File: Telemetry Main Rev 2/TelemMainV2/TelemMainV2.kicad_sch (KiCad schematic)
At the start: 19 parts, among them J1 8 pin ATM connector, J3 12 pin ATM connector, J4 SD to SPI (Molex nanofit), U3 NUCLEO-F446RE, U4 ISO1050DUB, U6 MCP6004

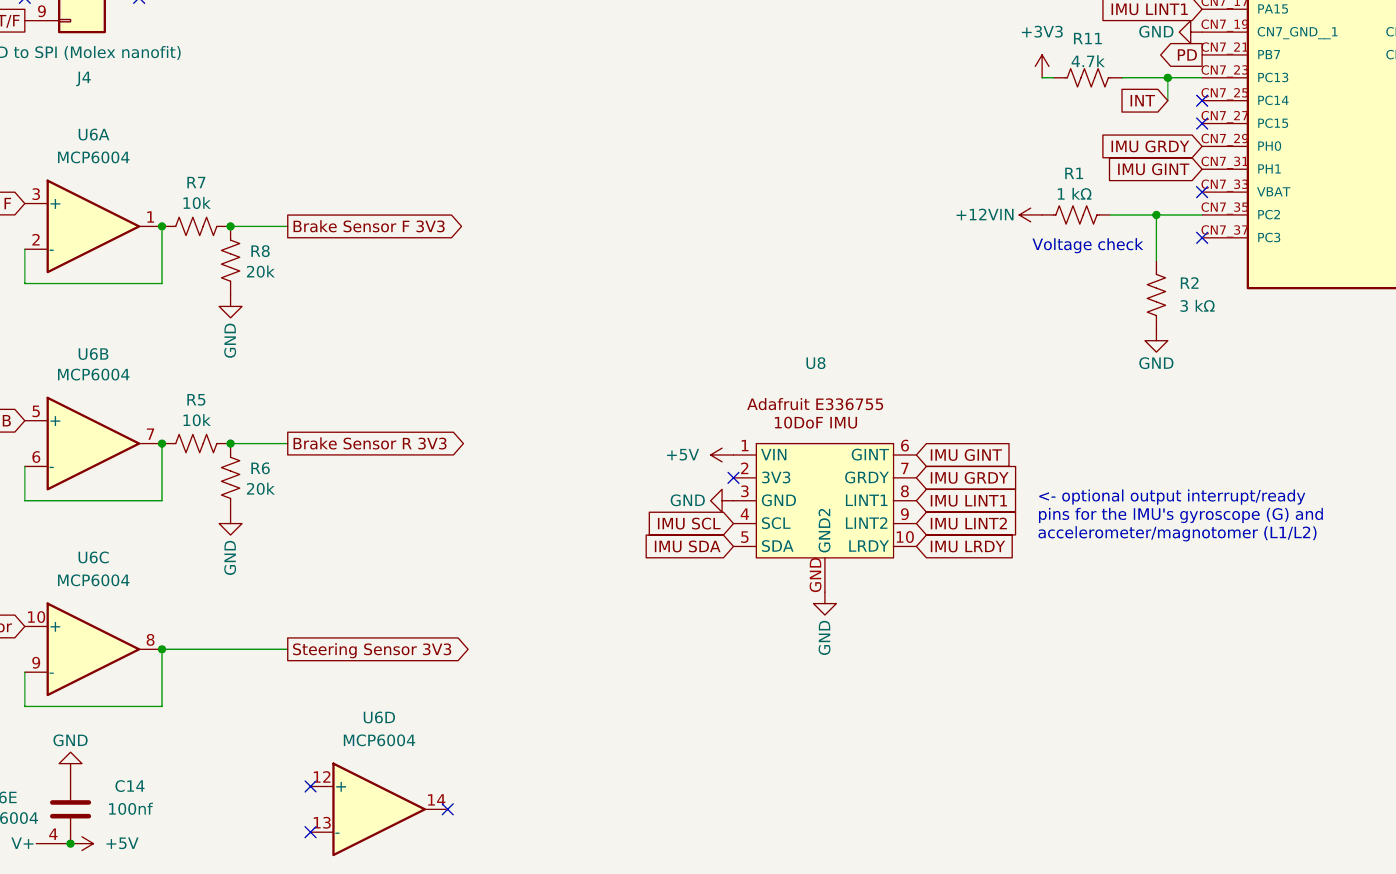
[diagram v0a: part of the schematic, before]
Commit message: stopped a micro pin from being blown up at a solid 9V
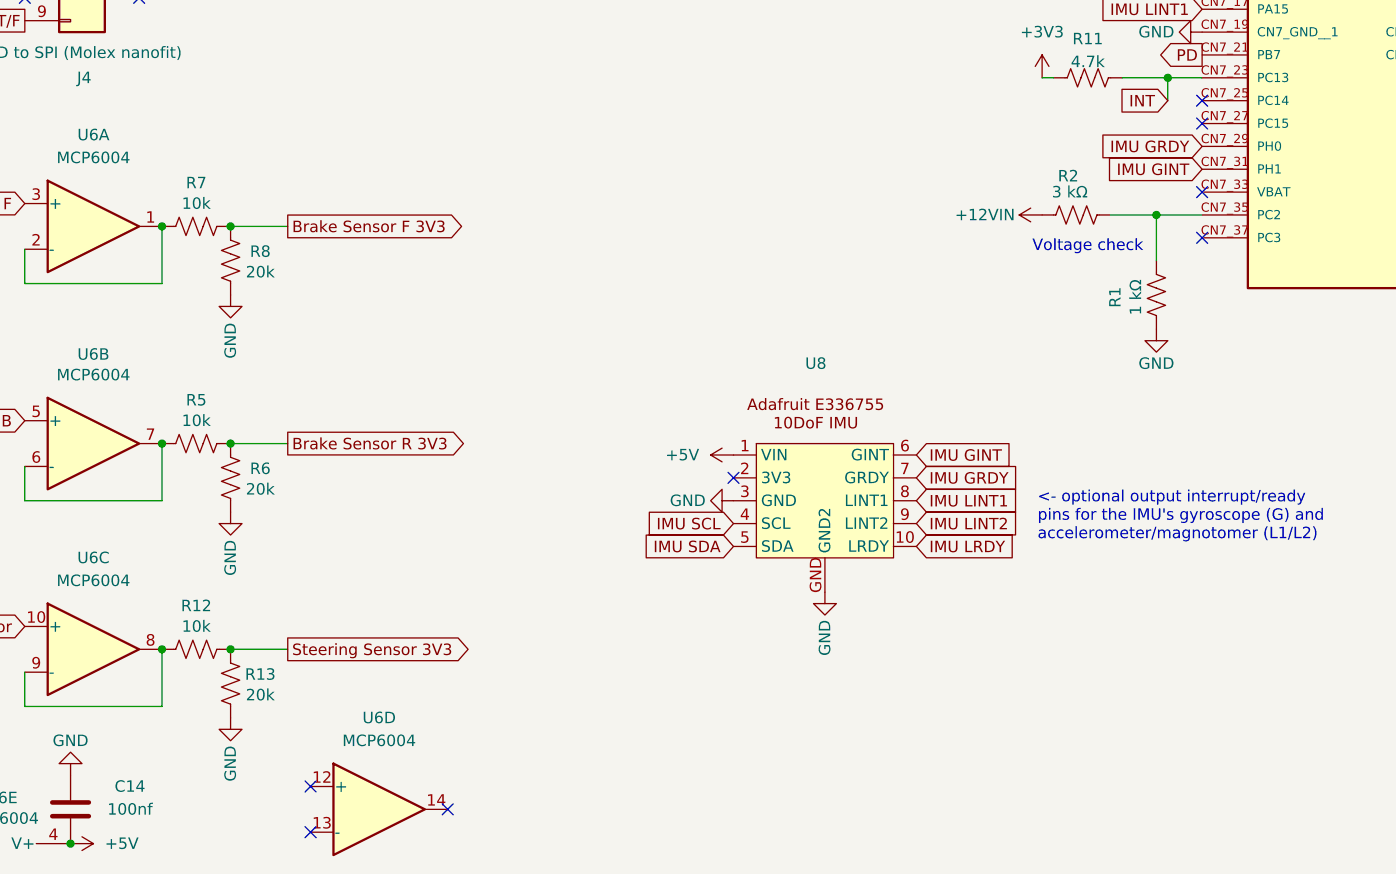
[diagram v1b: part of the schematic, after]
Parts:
- added R12: 10k, Resistor_SMD:R_0805_2012Metric_Pad1.20x1.40mm_HandSolder, symbol Device:R_US
- added R13: 20k, Resistor_SMD:R_0805_2012Metric_Pad1.20x1.40mm_HandSolder, symbol Device:R_US
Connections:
- net +12VIN: now also R2.2; no longer R1.1
- net GND: now also R1.1, R13.1; no longer R2.1
- net Steering Sensor 3V3: now also R12.2, R13.2; no longer U6.8, U6.9 (-)
- net at R1.2, U3.CN7_35 (PC2): now also R2.1; no longer R2.2
- new net: R12.1, U6.8, U6.9 (-)
